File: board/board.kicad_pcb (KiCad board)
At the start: 2 copper layers, 21 x 13 mm, 1 part

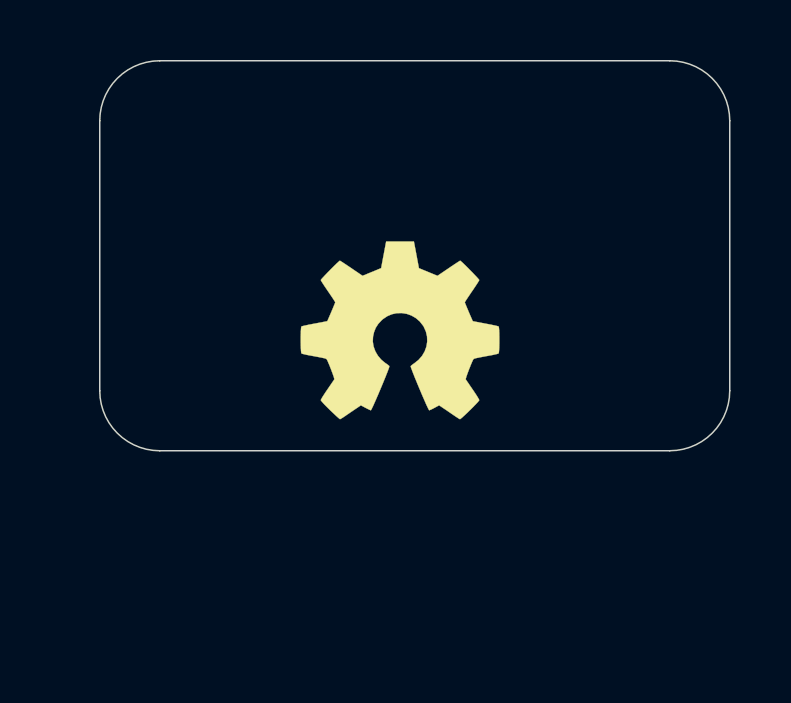
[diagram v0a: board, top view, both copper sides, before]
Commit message: initial
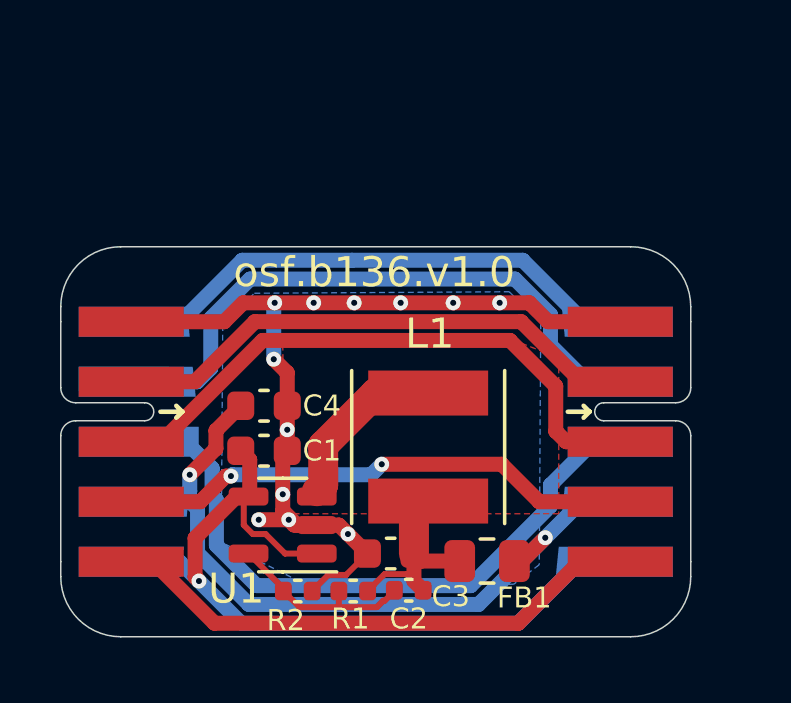
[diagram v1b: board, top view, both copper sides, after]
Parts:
- added C1: 22uF, Capacitor_SMD:C_0603_1608Metric, F.Cu at (145.5, 103.0)
- added C2: 22pF, Capacitor_SMD:C_0402_1005Metric, F.Cu at (150.3, 107.7)
- added C3: 22uF, Capacitor_SMD:C_0603_1608Metric, F.Cu at (149.7, 106.4)
- added C4: 22uF, Capacitor_SMD:C_0603_1608Metric, F.Cu at (145.5, 101.5)
- added FB1: 120R, Resistor_SMD:R_0805_2012Metric, F.Cu at (152.9, 106.7)
- added J1: 003_power, on_edge:on_edge_2x05_device, F.Cu at (138.7, 102.7)
- added J2: 003_power, on_edge:on_edge_2x05_host, F.Cu at (159.7, 102.7)
- added L1: 2.2uH, Inductor_SMD:L_Taiyo-Yuden_NR-50xx, F.Cu at (150.9, 102.9)
- added R1: 453k, Capacitor_SMD:C_0402_1005Metric, F.Cu at (148.4, 107.7)
- added R2: 100k, Capacitor_SMD:C_0402_1005Metric, F.Cu at (146.6, 107.7)
- added U1: AP3429, Package_TO_SOT_SMD:TSOT-23-5, F.Cu at (146.1, 105.5)
- LOGO1: moved to B.Cu
- moved LOGO1 3.85 mm to (148.9, 102.7), turned to 180 degrees
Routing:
- net GND: track 0.00 -> 31.8 mm, vias 0 -> 12
- net /dcdc_3.3v/in: track 0.00 -> 27.3 mm, vias 0 -> 1
- net /dcdc_3.3v/out: track 0.00 -> 26.8 mm, vias 0 -> 2
- net Net-(J1-Pad8): track 0.00 -> 21.9 mm
- net Net-(J1-Pad7): track 0.00 -> 21.0 mm
- net Net-(J1-Pad3): track 0.00 -> 20.0 mm
- net Net-(J1-Pad5): track 0.00 -> 18.0 mm
- net Net-(J1-Pad2): track 0.00 -> 18.0 mm
- net Net-(J1-Pad6): track 0.00 -> 17.9 mm
- net Net-(J1-Pad4): track 0.00 -> 17.3 mm, vias 0 -> 2
- net Net-(C2-Pad1): track 0.00 -> 6.80 mm
- net Net-(C2-Pad2): track 0.00 -> 6.44 mm
- net /dcdc_3.3v/LX: track 0.00 -> 5.84 mm
- added copper zone on F.Cu, net /dcdc_3.3v/LX
- added copper zone on B.Cu, net GND
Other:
- outline, holes or cut-outs redrawn
- board text added: "osf.b136.v1.0"
